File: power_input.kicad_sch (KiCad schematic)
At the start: 99 parts, among them J201 61300211121, J202 61300211121, J203 61300211121, J204 61300211121, J205 61300211121, J206 61300211121, J207 61300211121, J208 61300211121, Q201 SQ2319CES, Q202 SQ2319CES, Q203 IRFL4315TRPBF, Q204 SQ2319CES, Q205 SQ2319CES, U201 LM4040-5.0, U202 TL331, U203 OPA197, U204 LM4040-5.0, U205 TL331, U206 LM4040-5.0, U207 TL331

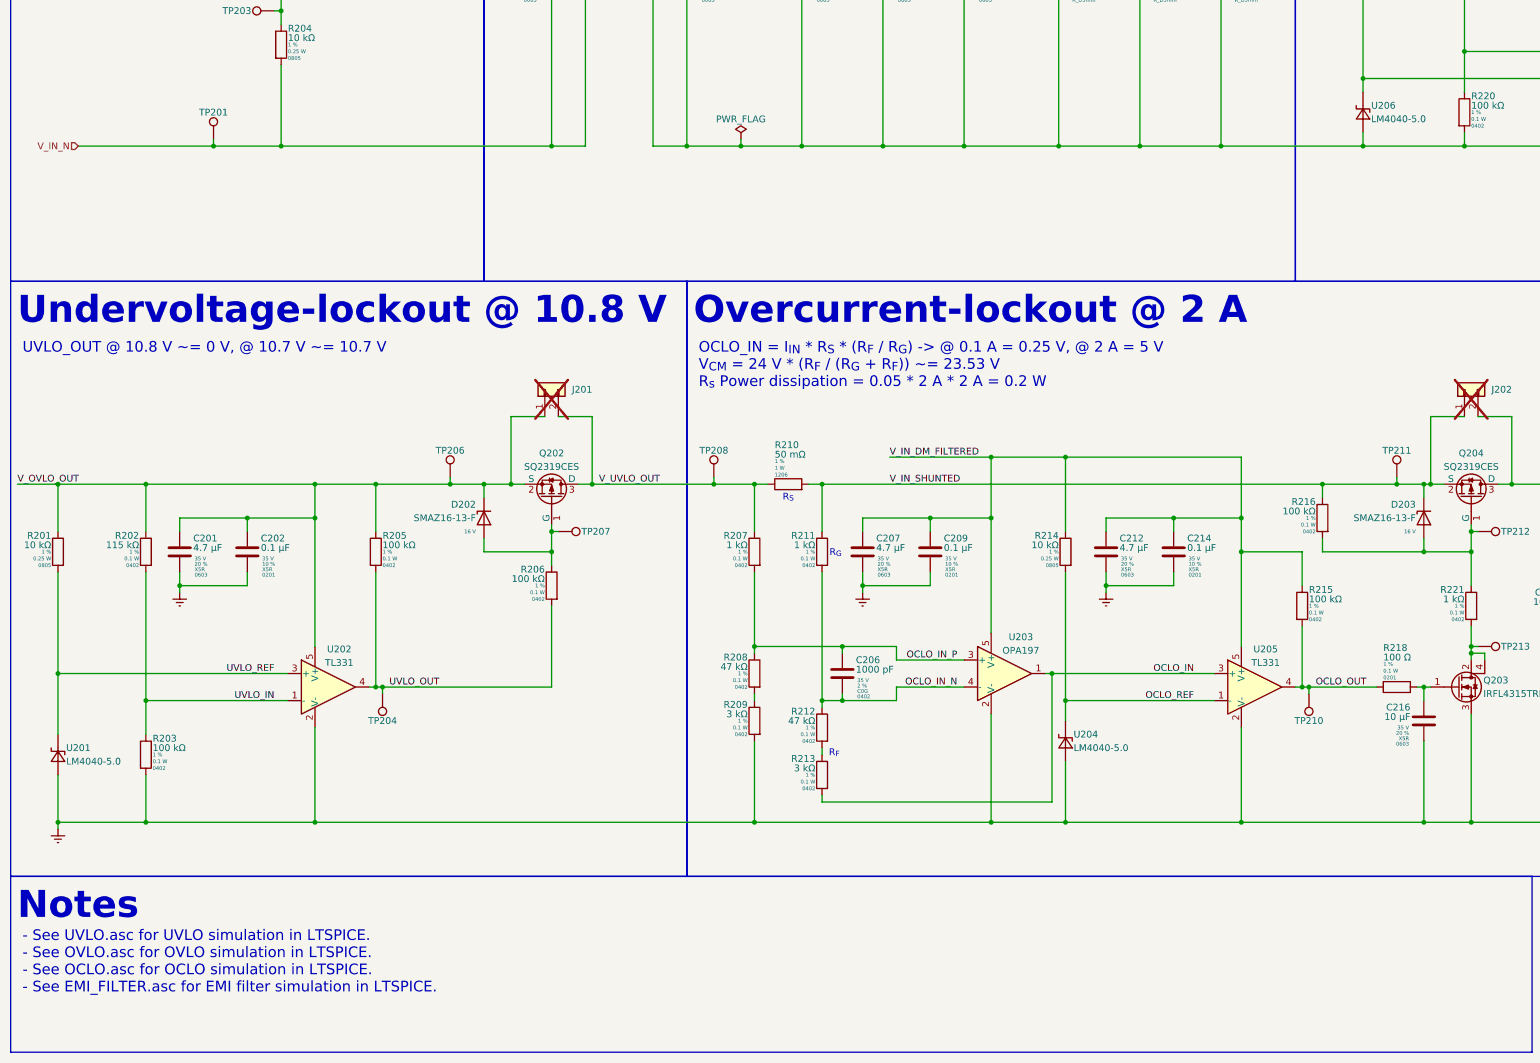
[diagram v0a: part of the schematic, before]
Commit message: Clean up schematics
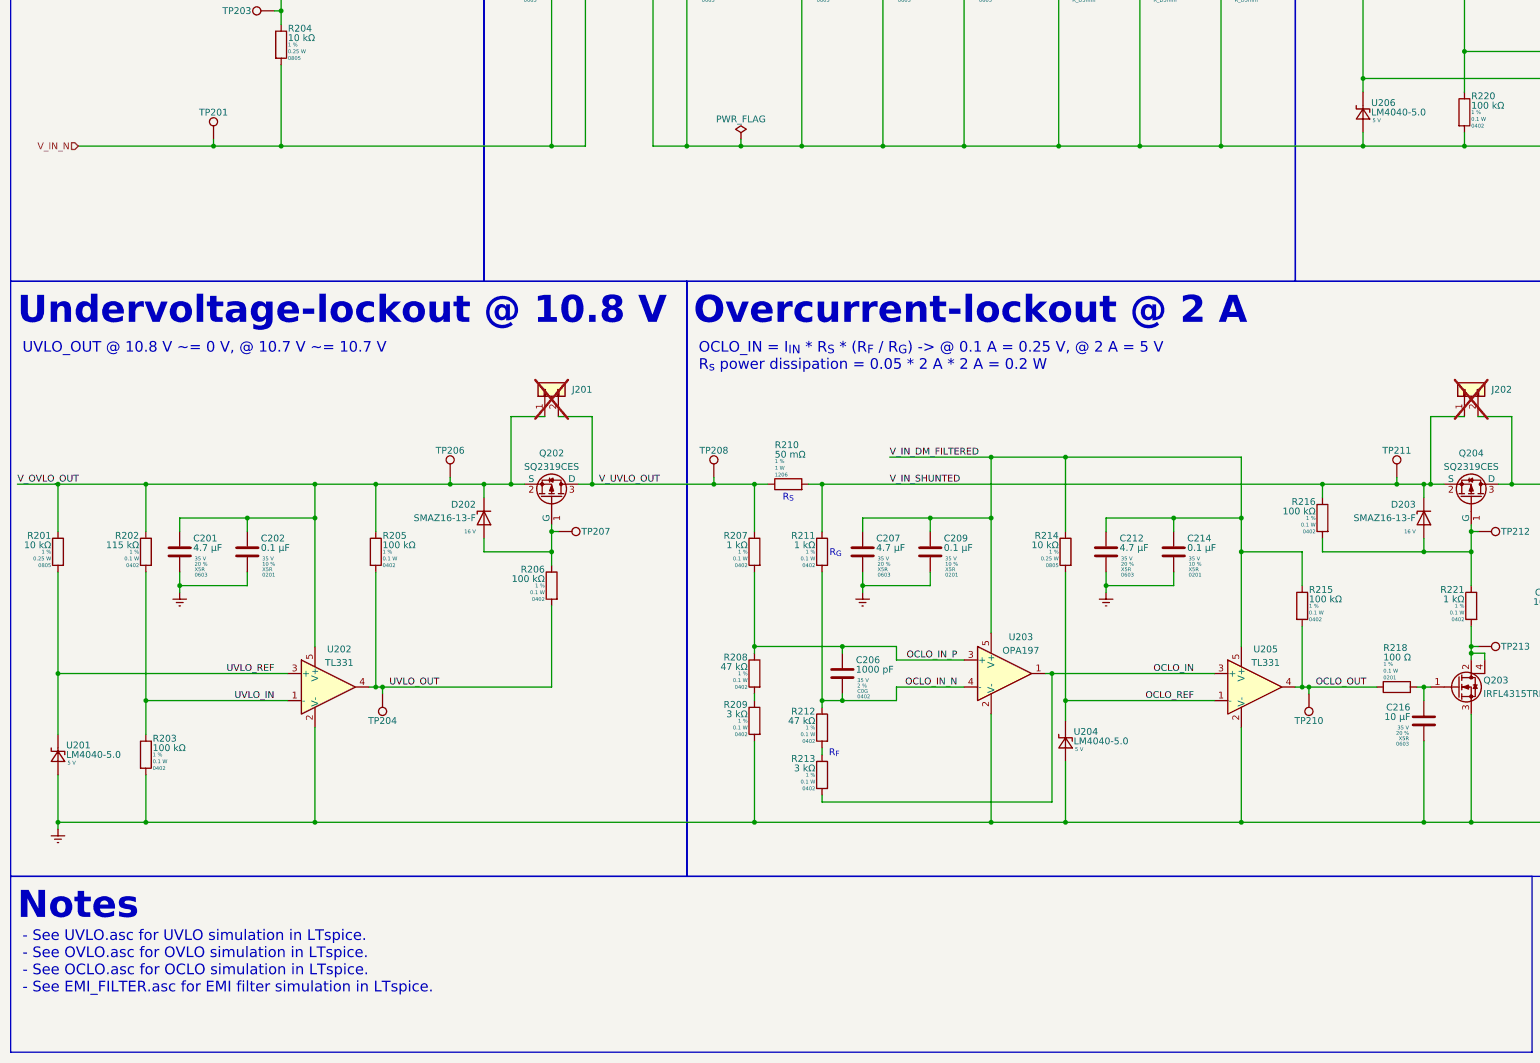
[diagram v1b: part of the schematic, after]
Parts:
- U201, U204, U206: Zener voltage (none) -> 5 V
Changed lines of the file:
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@@
 	(title_block
 		(title "Linux SBC")
-		(date "2025-12-19")
+		(date "2025-12-26")
 		(rev "v1.0.0")
 	)
@@
 		)
 	)
-	(text_box "- See UVLO.asc for UVLO simulation in LTSPICE.\n- See OVLO.asc for OVLO simulation in LTSPICE.\n- See OCLO.asc for OCLO simulation in LTSPICE.\n- See EMI_FILTER.asc for EMI filter simulation in LTSPICE."
+	(text_box "- See UVLO.asc for UVLO simulation in LTspice.\n- See OVLO.asc for OVLO simulation in LTspice.\n- See OCLO.asc for OCLO simulation in LTspice.\n- See EMI_FILTER.asc for EMI filter simulation in LTspice."
 		(exclude_from_sim no)
 		(at 13.97 260.35 0)
@@
 		)
 	)
-	(text_box "OCLO_IN = I_{IN} * R_{S} * (R_{F} / R_{G}) -> @ 0.1 A = 0.25 V, @ 2 A = 5 V\nV_{CM} = 24 V * (R_{F} / (R_{G} + R_{F})) ~= 23.53 V\nR_{s} Power dissipation = 0.05 * 2 A * 2 A = 0.2 W"
+	(text_box "OCLO_IN = I_{IN} * R_{S} * (R_{F} / R_{G}) -> @ 0.1 A = 0.25 V, @ 2 A = 5 V\nR_{s} power dissipation = 0.05 * 2 A * 2 A = 0.2 W"
 		(exclude_from_sim no)
 		(at 140.97 149.86 0)
@@
 		(dnp no)
 		(property "Reference" "U204"
-			(at 212.344 224.79 90)
+			(at 212.344 224.282 90)
 			(effects
 				(font
@@
 		)
 		(property "Value" "LM4040-5.0"
-			(at 212.344 227.33 90)
+			(at 212.344 226.06 90)
 			(effects
 				(font
@@
 			)
 		)
+		(property "Zener voltage" "5 V"
+			(at 212.598 227.584 90)
+			(effects
+				(font
+					(size 0.7 0.7)
+				)
+				(justify right)
+			)
+		)
 		(pin "2"
 		)
@@
 		(dnp no)
 		(property "Reference" "U206"
-			(at 268.224 106.68 90)
+			(at 268.224 106.172 90)
 			(effects
 				(font
@@
 		)
 		(property "Value" "LM4040-5.0"
-			(at 268.224 109.22 90)
+			(at 268.224 107.95 90)
 			(effects
 				(font
@@
 			)
 		)
+		(property "Zener voltage" "5 V"
+			(at 268.478 109.474 90)
+			(effects
+				(font
+					(size 0.7 0.7)
+				)
+				(justify right)
+			)
+		)
 		(pin "2"
 		)
@@
 	)
 	(symbol
+		(lib_id "Reference_Voltage:LM4040DBZ-5")
+		(at 21.59 228.6 90)
+		(unit 1)
+		(exclude_from_sim no)
+		(in_bom yes)
+		(on_board yes)
+		(dnp no)
+		(property "Reference" "U201"
+			(at 23.114 226.822 90)
+			(effects
+				(font
+					(size 1.27 1.27)
+				)
+				(justify right)
+			)
+		)
+		(property "Value" "LM4040-5.0"
+			(at 23.114 228.6 90)
+			(effects
+				(font
+					(size 1.27 1.27)
+				)
+				(justify right)
+			)
+		)
+		(property "Footprint" "Package_TO_SOT_SMD:SOT-23"
+			(at 26.67 228.6 0)
+			(effects
+				(font
+					(size 1.27 1.27)
+					(italic yes)
+				)
+				(hide yes)
+			)
+		)
+		(property "Datasheet" "https://ww1.microchip.com/downloads/aemDocuments/documents/OTH/ProductDocuments/DataSheets/LM4040-41-Precision-Micropower-Shunt-Voltage-Reference-DS20005757B.pdf"
+			(at 21.59 228.6 0)
+			(effects
+				(font
+					(size 1.27 1.27)
+					(italic yes)
+				)
+				(hide yes)
+			)
+		)
+		(property "Description" "Shunt Voltage Reference IC Fixed 5V V ±1% 15 mA SOT-23-3"
+			(at 21.59 228.6 0)
+			(effects
+				(font
+					(size 1.27 1.27)
+				)
+				(hide yes)
+			)
+		)
+		(property "Digi-Key Part Number" "576-2570-1-ND"
+			(at 21.59 228.6 90)
+			(effects
+				(font
+					(size 1.27 1.27)
+				)
+				(hide yes)
+			)
+		)
+		(property "MPN" "LM4040DYM3-5.0-TR"
+			(at 21.59 228.6 90)
+			(effects
+				(font
+					(size 1.27 1.27)
+				)
+				(hide yes)
+			)
+		)
+		(property "Manufacturer" "Microchip Technology"
+			(at 21.59 228.6 90)
+			(effects
+				(font
+					(size 1.27 1.27)
+				)
+				(hide yes)
+			)
+		)
+		(property "Zener voltage" "5 V"
+			(at 23.368 230.124 90)
+			(effects
+				(font
+					(size 0.7 0.7)
+				)
+				(justify right)
+			)
+		)
+		(pin "2"
+		)
+		(pin "3"
+		)
+		(pin "1"
+		)
+		(instances
+			(project "linux-sbc"
+				(path "/fa11a02f-8043-4153-ab69-88d766503017/524a017a-f4b1-440b-9b41-00cccec69d8d"
+					(reference "U201")
+					(unit 1)
+				)
+			)
+		)
+	)
+	(symbol
 		(lib_id "Connector:TestPoint")
 		(at 62.23 88.9 90)
@@
 					(unit 1)
 				)
-			)
-		)
-	)
-	(symbol
-		(lib_name "LM4040DBZ-5_1")
-		(lib_id "Reference_Voltage:LM4040DBZ-5")
-		(at 21.59 228.6 90)
-		(unit 1)
-		(exclude_from_sim no)
-		(in_bom yes)
-		(on_board yes)
-		(dnp no)
-		(property "Reference" "U201"
-			(at 23.114 227.33 90)
-			(effects
-				(font
-					(size 1.27 1.27)
-				)
-				(justify right)
-			)
-		)
-		(property "Value" "LM4040-5.0"
-			(at 23.114 229.87 90)
-			(effects
-				(font
-					(size 1.27 1.27)
-				)
-				(justify right)
-			)
-		)
-		(property "Footprint" "Package_TO_SOT_SMD:SOT-23"
-			(at 26.67 228.6 0)
-			(effects
-				(font
-					(size 1.27 1.27)
-					(italic yes)
-				)
-				(hide yes)
-			)
-		)
-		(property "Datasheet" "https://ww1.microchip.com/downloads/aemDocuments/documents/OTH/ProductDocuments/DataSheets/LM4040-41-Precision-Micropower-Shunt-Voltage-Reference-DS20005757B.pdf"
-			(at 21.59 228.6 0)
-			(effects
-				(font
-					(size 1.27 1.27)
-					(italic yes)
-				)
-				(hide yes)
-			)
-		)
-		(property "Description" "Shunt Voltage Reference IC Fixed 5V V ±1% 15 mA SOT-23-3"
-			(at 21.59 228.6 0)
-			(effects
-				(font
-					(size 1.27 1.27)
-				)
-				(hide yes)
-			)
-		)
-		(property "Digi-Key Part Number" "576-2570-1-ND"
-			(at 21.59 228.6 90)
-			(effects
-				(font
-					(size 1.27 1.27)
-				)
-				(hide yes)
-			)
-		)
-		(property "MPN" "LM4040DYM3-5.0-TR"
-			(at 21.59 228.6 90)
-			(effects
-				(font
-					(size 1.27 1.27)
-				)
-				(hide yes)
-			)
-		)
-		(property "Manufacturer" "Microchip Technology"
-			(at 21.59 228.6 90)
-			(effects
-				(font
-					(size 1.27 1.27)
-				)
-				(hide yes)
-			)
-		)
-		(pin "2"
-		)
-		(pin "3"
-		)
-		(pin "1"
-		)
-		(instances
-			(project "linux-sbc"
-				(path "/fa11a02f-8043-4153-ab69-88d766503017/524a017a-f4b1-440b-9b41-00cccec69d8d"
-					(reference "U201")
-					(unit 1)
-				)
